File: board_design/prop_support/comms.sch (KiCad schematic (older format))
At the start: 17 parts, among them J4 USB_B, U6 FT232H, Y1 CX3225CA

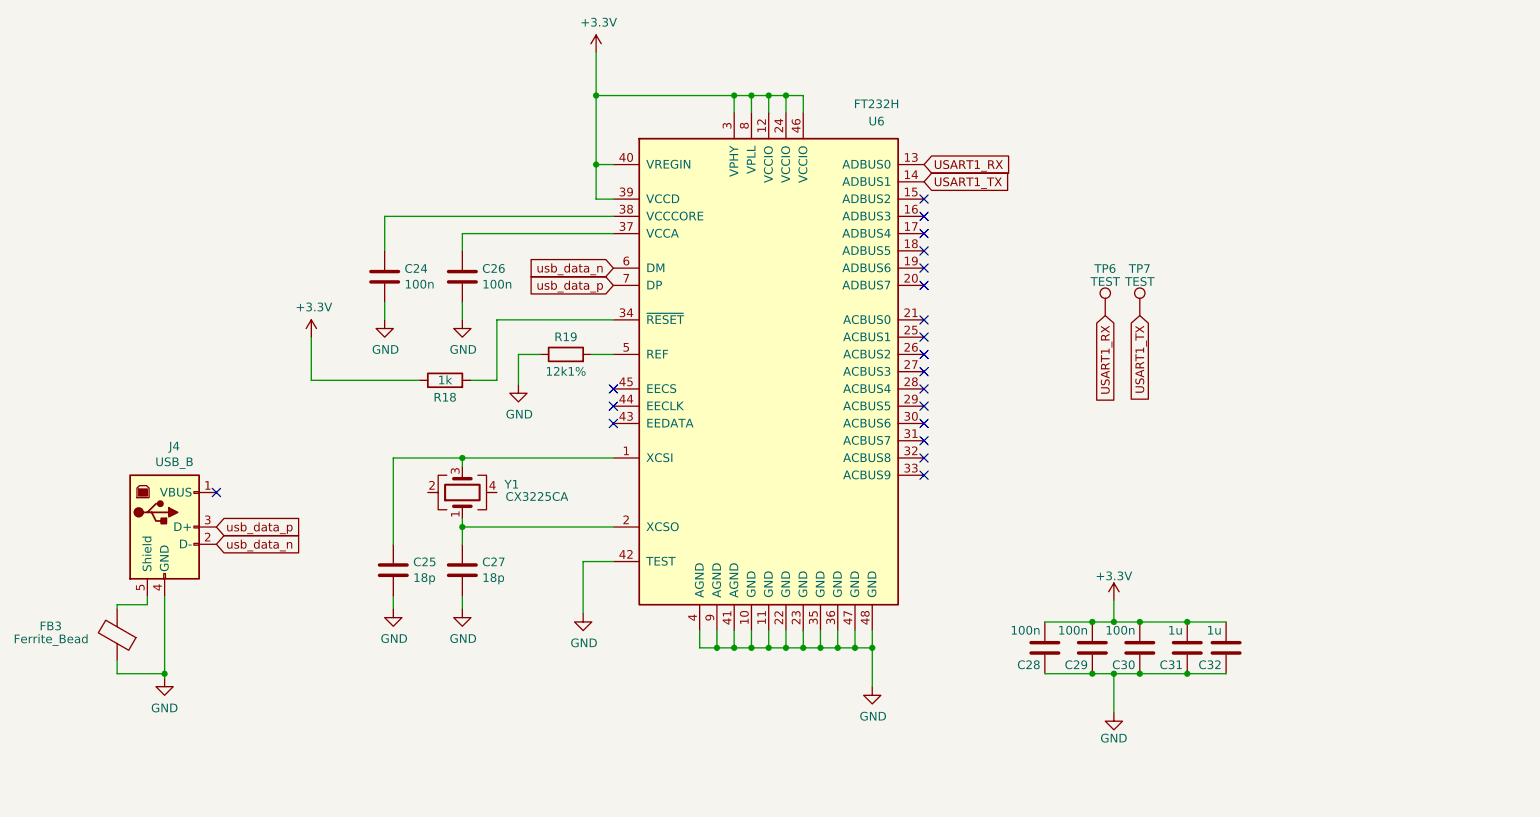
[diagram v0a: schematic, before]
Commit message: first MX export
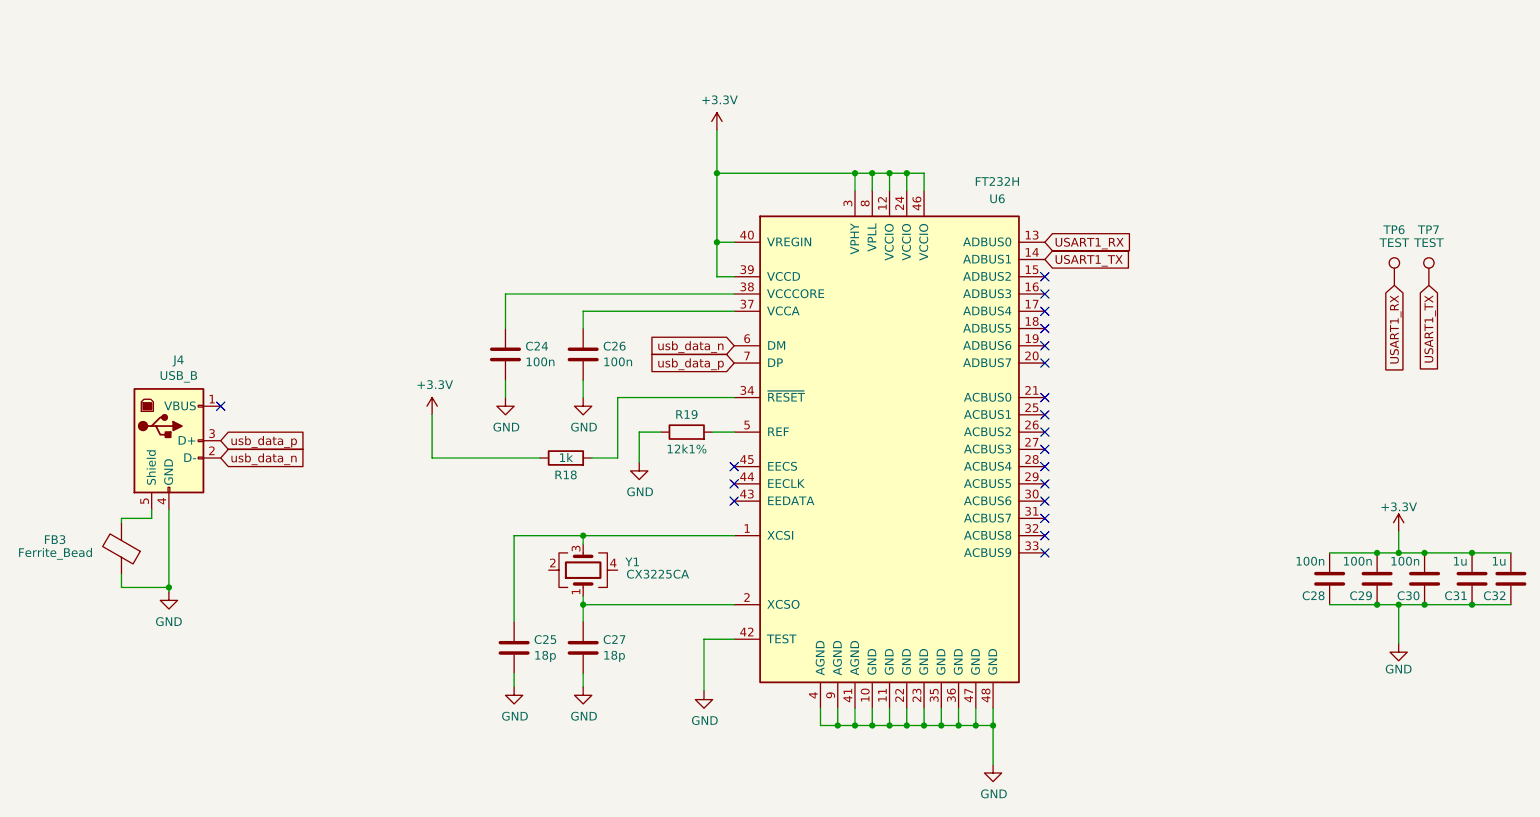
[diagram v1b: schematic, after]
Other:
- moved on the sheet: C24, C25, C26, C27, C28, C29, C30, C31, C32, FB3, J4, R18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
